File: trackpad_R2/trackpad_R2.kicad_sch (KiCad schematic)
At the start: 41 parts, among them U1 74HC4051, U2 74HC4051, U3 74HC4051, U4 STM32F303CCTx, U5 LM1117MP-3.3, U6 74HC4051, Y1 8MHz

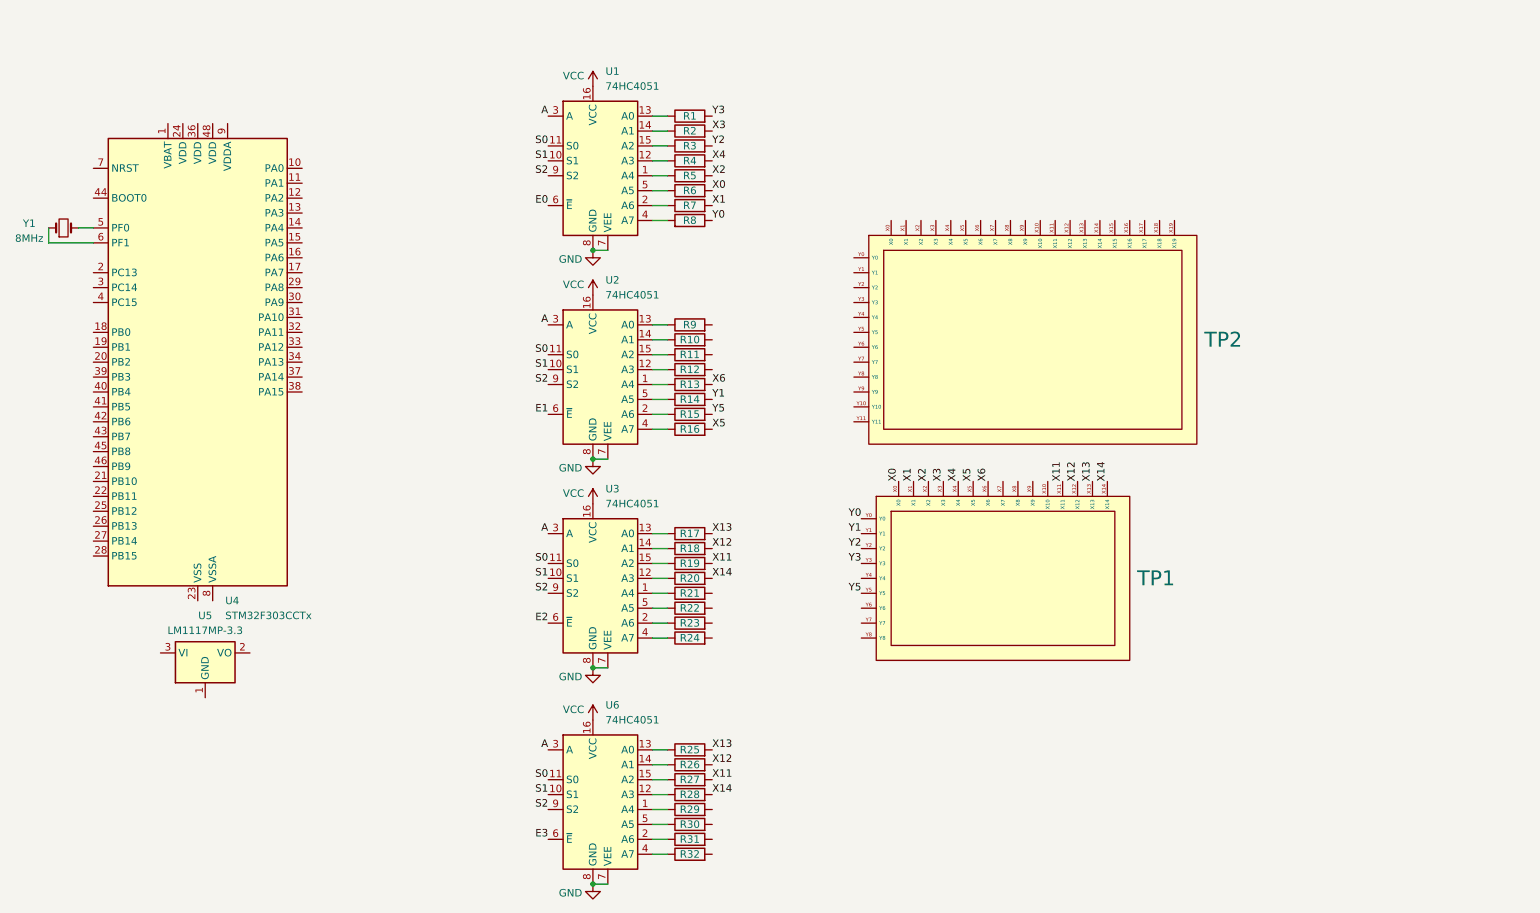
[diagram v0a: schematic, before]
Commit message: progres
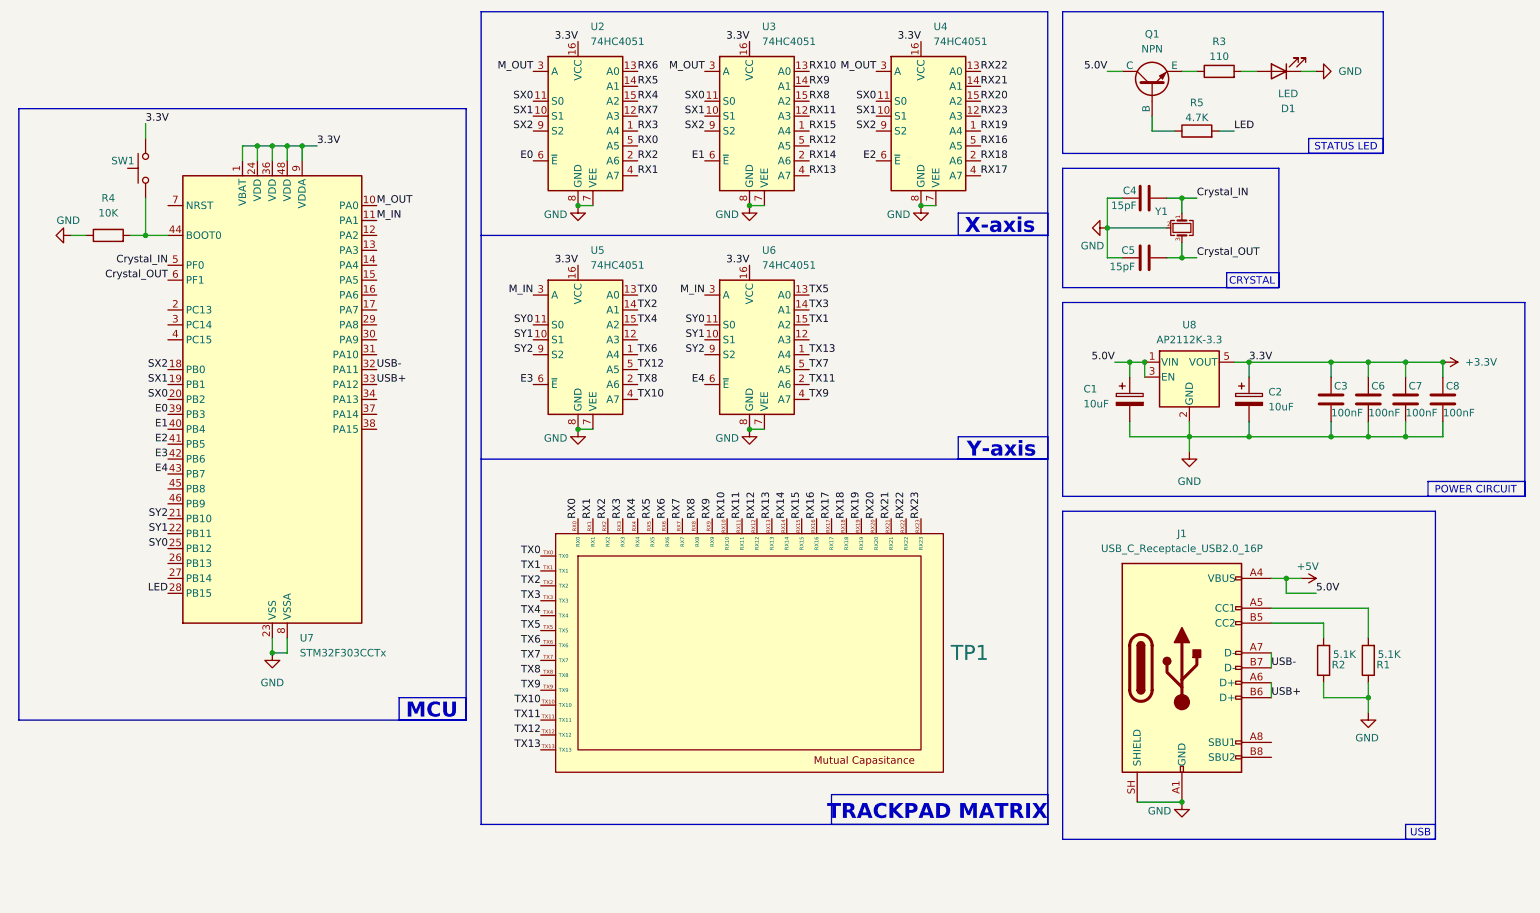
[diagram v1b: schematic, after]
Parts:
- removed R10, R11, R12, R13, R14, R15, R16, R17, R18, R19, R20, R21, R22, R23, R24, R25, R26, R27, R28, R29, R30, R31, R32, R6, R7, R8, R9: R, Resistor_SMD:R_0805_2012Metric_Pad1.20x1.40mm_HandSolder, symbol Device:R
- removed TP1: (no value), symbol symboleita:trackpad_15x9
- removed TP2: (no value), trackpads:trackpad_20x12_130mm_78mm, symbol symboleita:trackpad_20x12
- removed U5: LM1117MP-3.3, Package_TO_SOT_SMD:SOT-223-3_TabPin2, symbol Regulator_Linear:LM1117MP-3.3
- removed Y1: 8MHz, Oscillator:Oscillator_DIP-14, symbol Device:Crystal_Small
- added C1, C2: 10uF, Capacitor_SMD:C_0805_2012Metric, symbol Device:C_Polarized
- added C3, C6, C7, C8: 100nF, Capacitor_SMD:C_0603_1608Metric_Pad1.08x0.95mm_HandSolder, symbol Device:C
- added C4, C5: 15pF, Capacitor_SMD:C_0603_1608Metric_Pad1.08x0.95mm_HandSolder, symbol Device:C
- added D1: LED, LED_SMD:LED_1206_3216Metric_ReverseMount_Hole1.8x2.4mm, symbol Device:LED
- added J1: USB_C_Receptacle_USB2.0_16P, Connector_USB:USB_C_Receptacle_GCT_USB4105-xx-A_16P_TopMnt_Horizontal, symbol Connector:USB_C_Receptacle_USB2.0_16P
- added Q1: NPN, Package_TO_SOT_SMD:SOT-323_SC-70, symbol Simulation_SPICE:NPN
- added SW1: SW_Omron_B3FS, Button_Switch_SMD:SW_Push_1P1T_NO_CK_KMR2, symbol Switch:SW_Omron_B3FS
- added TP1: (no value), trackpads:trackpad_24x14_132mm_77mm, symbol symboleita:trackpad_24x14
- added U4: 74HC4051, Package_SO:SOIC-16_3.9x9.9mm_P1.27mm, symbol 74xx:74HC4051
- added U8: AP2112K-3.3, Package_TO_SOT_SMD:SOT-23-5, symbol Regulator_Linear:AP2112K-3.3
- added Y1: Crystal, Crystal:Crystal_SMD_Abracon_ABM8G-4Pin_3.2x2.5mm, symbol Device:Crystal_GND24_Small
- R1, R2: value R -> 5.1K; footprint Resistor_SMD:R_0805_2012Metric_Pad1.20x1.40mm_HandSolder -> Resistor_SMD:R_0603_1608Metric_Pad0.98x0.95mm_HandSolder
- R3: value R -> 110; footprint Resistor_SMD:R_0805_2012Metric_Pad1.20x1.40mm_HandSolder -> Resistor_SMD:R_0603_1608Metric_Pad0.98x0.95mm_HandSolder
- R4: value R -> 10K; footprint Resistor_SMD:R_0805_2012Metric_Pad1.20x1.40mm_HandSolder -> Resistor_SMD:R_0603_1608Metric_Pad0.98x0.95mm_HandSolder
- R5: value R -> 4.7K; footprint Resistor_SMD:R_0805_2012Metric_Pad1.20x1.40mm_HandSolder -> Resistor_SMD:R_0603_1608Metric_Pad0.98x0.95mm_HandSolder
- renumbered U1 to U2, U2 to U3, U3 to U5, U4 to U7
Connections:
- net VCC is gone; now on net +3.3V: U2.16 (VCC), U3.16 (VCC), U5.16 (VCC), U6.16 (VCC)
- net X2 is gone; now on net LED: R5.2
- net X4 is gone; now on an unnamed net: R4.2
- net E0: now also U7.39 (PB3)
- net E1: now also U7.40 (PB4)
- net E2: now also U7.41 (PB5), U4.6 (~{E}); no longer U5.6 (~{E})
- net E3: now also U5.6 (~{E}), U7.42 (PB6); no longer U6.6 (~{E})
- net GND: now also R1.1, R2.1, R4.1, U7.23 (VSS), U7.35 (VSS), U7.47 (VSS), U7.8 (VSSA), C1.2, C2.2, C3.2, C4.1, C5.1, C6.2, C7.2, C8.2, D1.1 (K), J1.A1 (GND), J1.A12 (GND), J1.B1 (GND), J1.B12 (GND), J1.SH (SHIELD), U4.7 (VEE), U4.8 (GND), U8.2 (GND), Y1.2 (G), Y1.4 (G)
- net TX11: now reaches U6.2 (A6)
- net TX11: now also TP1.TX11
- net RX14: now reaches U3.2 (A6)
- net RX14: now also TP1.RX14
- net RX13: now reaches U3.4 (A7)
- net RX13: now also TP1.RX13
- net at R5.1: now also Q1.2 (B); no longer U2.1 (A4)
- net RX7: now reaches U2.12 (A3)
- net RX7: now also TP1.RX7; no longer R4.1
- net RX6: now reaches U2.13 (A0)
- net RX6: now also TP1.RX6; no longer R1.1
- net RX5: now reaches U2.14 (A1)
- net RX5: now also TP1.RX5; no longer R2.1
- net at R3.1: now also Q1.3 (E); no longer U2.15 (A2)
- net RX2: now reaches U2.2 (A6)
- net RX2: now also TP1.RX2
- net RX1: now reaches U2.4 (A7)
- net RX1: now also TP1.RX1
- net RX0: now reaches U2.5 (A5)
- net RX0: now also TP1.RX0
- net RX8: now reaches U3.15 (A2)
- net RX8: now also TP1.RX8
- net TX13: now reaches U6.1 (A4)
- net TX13: now also TP1.TX13
- net TX12: now reaches U5.5 (A5)
- net TX12: now also TP1.TX12
- net RX9: now reaches U3.14 (A1)
- net RX9: now also TP1.RX9
- net Crystal_OUT: now reaches U7.6 (PF1)
- net Crystal_OUT: now also C5.2, Y1.3
- net Crystal_IN: now reaches U7.5 (PF0)
- net Crystal_IN: now also C4.2, Y1.1
- net TX7: now reaches U6.5 (A5)
- net TX7: now also TP1.TX7
- net TX4: now reaches U5.15 (A2)
- net TX4: now also TP1.TX4
- net TX10: now reaches U5.4 (A7)
- net TX10: now also TP1.TX10
- net TX6: now reaches U5.1 (A4)
- net TX6: now also TP1.TX6
- net TX0: now reaches U5.13 (A0)
- net TX0: now also TP1.TX0
- net TX2: now reaches U5.14 (A1)
- net TX2: now also TP1.TX2
- net TX8: now reaches U5.2 (A6)
- net TX8: now also TP1.TX8
- net TX5: now reaches U6.13 (A0)
- net TX5: now also TP1.TX5
- net TX3: now reaches U6.14 (A1)
- net TX3: now also TP1.TX3
- net TX1: now reaches U6.15 (A2)
- net TX1: now also TP1.TX1
- net TX9: now reaches U6.4 (A7)
- net TX9: now also TP1.TX9
- net RX11: now reaches U3.12 (A3)
- net RX11: now also TP1.RX11
- net +3.3V: now reaches U7.1 (VBAT)
- net +3.3V: now also U7.24 (VDD), U7.36 (VDD), U7.48 (VDD), U7.9 (VDDA), C2.1, C3.1, C6.1, C7.1, C8.1, SW1.2, U4.16 (VCC), U8.5 (VOUT)
- net M_OUT: now reaches U7.10 (PA0)
- net M_OUT: now also U2.3 (A), U3.3 (A), U4.3 (A)
- net M_IN: now reaches U7.11 (PA1)
- net M_IN: now also U5.3 (A), U6.3 (A)
- net SX2: now reaches U7.18 (PB0)
- net SX2: now also U2.9 (S2), U3.9 (S2), U4.9 (S2)
- net SX1: now reaches U7.19 (PB1)
- net SX1: now also U2.10 (S1), U3.10 (S1), U4.10 (S1)
- net SX0: now reaches U7.20 (PB2)
- net SX0: now also U2.11 (S0), U3.11 (S0), U4.11 (S0)
- net SY2: now reaches U7.21 (PB10)
- net SY2: now also U5.9 (S2), U6.9 (S2)
- net SY1: now reaches U7.22 (PB11)
- net SY1: now also U5.10 (S1), U6.10 (S1)
- net SY0: now reaches U7.25 (PB12)
- net SY0: now also U5.11 (S0), U6.11 (S0)
- net LED: now reaches U7.28 (PB15)
- net USB-: now reaches U7.32 (PA11)
- net USB-: now also J1.A7 (D-), J1.B7 (D-)
- net USB+: now reaches U7.33 (PA12)
- net USB+: now also J1.A6 (D+), J1.B6 (D+)
- net E4: now reaches U7.43 (PB7)
- net E4: now also U6.6 (~{E})
- net at U7.44 (BOOT0): now also SW1.1
- net RX15: now reaches U3.1 (A4)
- net RX15: now also TP1.RX15
- net RX10: now reaches U3.13 (A0)
- net RX10: now also TP1.RX10
- net RX12: now reaches U3.5 (A5)
- net RX12: now also TP1.RX12
- removed net A: U2.3 (A), U3.3 (A), U5.3 (A), U6.3 (A)
- removed net S0: U2.11 (S0), U3.11 (S0), U5.11 (S0), U6.11 (S0)
- removed net S1: U2.10 (S1), U3.10 (S1), U5.10 (S1), U6.10 (S1)
- removed net S2: U2.9 (S2), U3.9 (S2), U5.9 (S2), U6.9 (S2)
- net X3: no longer names the net of R2.2
- net X3: now also J1.B5 (CC2)
- net Y2: no longer names the net of R3.2
- net Y2: now also D1.2 (A)
- net Y3: no longer names the net of R1.2
- net Y3: now also J1.A5 (CC1)
- new net +5V: C1.1, J1.A4 (VBUS), J1.A9 (VBUS), J1.B4 (VBUS), J1.B9 (VBUS), Q1.1 (C), U8.1 (VIN), U8.3 (EN)
- new net RX16: TP1.RX16, U4.5 (A5)
- new net RX17: TP1.RX17, U4.4 (A7)
- new net RX18: TP1.RX18, U4.2 (A6)
- new net RX19: TP1.RX19, U4.1 (A4)
- new net RX20: TP1.RX20, U4.15 (A2)
- new net RX21: TP1.RX21, U4.14 (A1)
- new net RX22: TP1.RX22, U4.13 (A0)
- new net RX23: TP1.RX23, U4.12 (A3)
- new net RX3: TP1.RX3, U2.1 (A4)
- new net RX4: TP1.RX4, U2.15 (A2)
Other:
- note added: "CRYSTAL"
- note added: "MCU"
- note added: "POWER CIRCUIT"
- note added: "STATUS LED"
- note added: "TRACKPAD MATRIX"
- note added: "USB"
- note added: "X-axis"
- note added: "Y-axis"
- moved on the sheet: U2, U3, U5, U6, U7
